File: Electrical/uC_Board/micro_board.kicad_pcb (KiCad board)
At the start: 2 copper layers, 45 x 18 mm, 27 parts, among them J1 card_edge_6p, SW1 SW_Push, U1 ATmega328PB-AU, U2 ArdStripNano, U3 CSTNE16M0V530000R0, U4 AD8620, U5 LM1117MPX-5.0

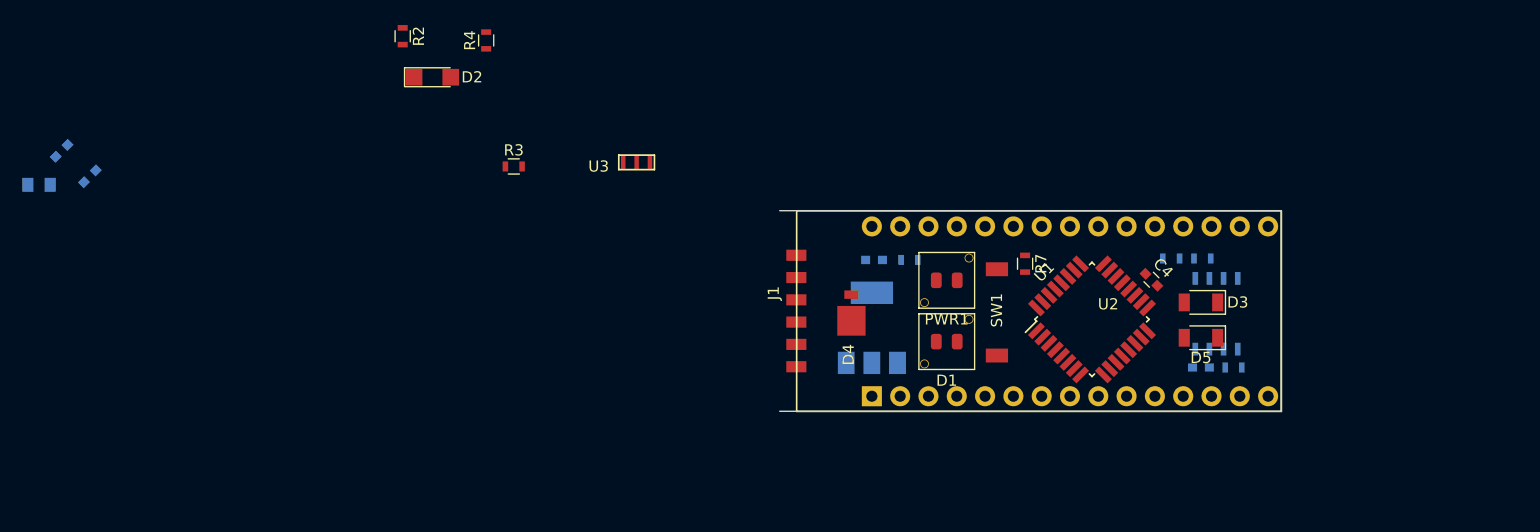
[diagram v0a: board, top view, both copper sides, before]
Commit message: forgot to save earlier
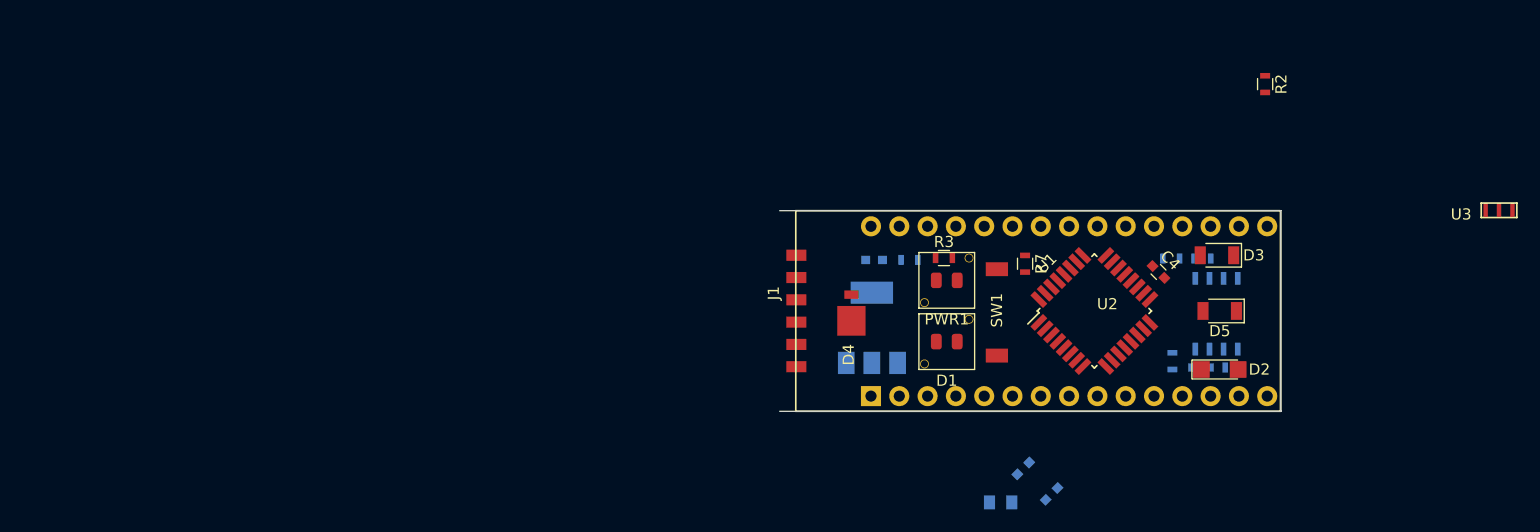
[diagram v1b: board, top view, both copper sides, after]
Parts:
- R4: moved to B.Cu
- moved C1 90.9 mm to (124.4, 116.4)
- moved C2 90.9 mm to (119.8, 117.2)
- moved C3 90.9 mm to (121.9, 114.1)
- moved R2 77.5 mm to (143.6, 79.6)
- moved U3 77.5 mm to (163.0, 91.6)
- moved D2 75.4 mm to (139.5, 105.2)
- moved R4 68.0 mm to (135.2, 104.5), turned to 270 degrees
- moved R3 39.5 mm to (114.8, 95.2)
- moved D3 4.47 mm to (139.2, 95.0)
- moved D5 2.94 mm to (139.5, 100.0)
- moved C4 0.94 mm to (134.0, 96.5)
- moved U1 0.78 mm to (128.2, 100.0)
- moved U2 0.08 mm to (147.7, 91.0)
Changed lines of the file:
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@@
   (general
     (thickness 1.6)
-    (drawings 5)
+    (drawings 6)
     (tracks 0)
     (zones 0)
@@
   (layers
     (0 F.Cu signal)
-    (31 B.Cu signal)
+    (31 B.Cu signal hide)
     (32 B.Adhes user)
     (33 F.Adhes user)
@@
     (add_net VCC)
   )
-  (module hodgkin:LED_0805_LightPipe (layer F.Cu)
+  (module hodgkin:LED_0805_LightPipe locked (layer F.Cu)
     (at 115 97.25 180)
     (descr "LED SMD 1206 (3216 Metric), square (rectangular) end terminal, IPC_7351 nominal, (Body size source: http://www.tortai-tech.com/upload/download/2011102023233369053.pdf), generated with kicad-footprint-generator")
@@
     )
   )
-  (module hodgkin:LED_0805_LightPipe (layer F.Cu)
+  (module hodgkin:LED_0805_LightPipe locked (layer F.Cu)
     (at 115 102.75 180)
     (descr "LED SMD 1206 (3216 Metric), square (rectangular) end terminal, IPC_7351 nominal, (Body size source: http://www.tortai-tech.com/upload/download/2011102023233369053.pdf), generated with kicad-footprint-generator")
@@
   )
   (module hodgkin:CSTNE16M0V530000R0 (layer F.Cu)
-    (at 85.564999 87.313)
+    (at 162.964999 91.613)
     (fp_text reference U3 (at -1.802999 -0.285) (layer F.SilkS)
       (effects (font (size 1 1) (thickness 0.15)))
@@
       (net 31 "Net-(U1-Pad8)"))
   )
-  (module hodgkin:PTS636-G-2.5-NoGND (layer F.Cu)
+  (module hodgkin:PTS636-G-2.5-NoGND locked (layer F.Cu)
     (at 119.5 104 90)
     (fp_text reference SW1 (at 4.064 0 90) (layer F.SilkS)
@@
     )
   )
-  (module Resistors_SMD:R_0603 (layer F.Cu)
-    (at 73.666 75.722 90)
+  (module Resistors_SMD:R_0603 (layer B.Cu)
+    (at 135.25 104.5 270)
     (descr "Resistor SMD 0603, reflow soldering, Vishay (see dcrcw.pdf)")
     (tags "resistor 0603")
     (attr smd)
-    (fp_text reference R4 (at 0 -1.45 90) (layer F.SilkS)
-      (effects (font (size 1 1) (thickness 0.15)))
-    )
-    (fp_text value R (at 0 1.5 90) (layer F.Fab)
-      (effects (font (size 1 1) (thickness 0.15)))
-    )
-    (fp_text user %R (at 0 0 90) (layer F.Fab)
-      (effects (font (size 0.4 0.4) (thickness 0.075)))
-    )
-    (fp_line (start -0.8 0.4) (end -0.8 -0.4) (layer F.Fab) (width 0.1))
-    (fp_line (start 0.8 0.4) (end -0.8 0.4) (layer F.Fab) (width 0.1))
-    (fp_line (start 0.8 -0.4) (end 0.8 0.4) (layer F.Fab) (width 0.1))
-    (fp_line (start -0.8 -0.4) (end 0.8 -0.4) (layer F.Fab) (width 0.1))
-    (fp_line (start 0.5 0.68) (end -0.5 0.68) (layer F.SilkS) (width 0.12))
-    (fp_line (start -0.5 -0.68) (end 0.5 -0.68) (layer F.SilkS) (width 0.12))
-    (fp_line (start -1.25 -0.7) (end 1.25 -0.7) (layer F.CrtYd) (width 0.05))
-    (fp_line (start -1.25 -0.7) (end -1.25 0.7) (layer F.CrtYd) (width 0.05))
-    (fp_line (start 1.25 0.7) (end 1.25 -0.7) (layer F.CrtYd) (width 0.05))
-    (fp_line (start 1.25 0.7) (end -1.25 0.7) (layer F.CrtYd) (width 0.05))
-    (pad 1 smd rect (at -0.75 0 90) (size 0.5 0.9) (layers F.Cu F.Paste F.Mask)
+    (fp_text reference R4 (at 0 1.45 270) (layer B.SilkS)
+      (effects (font (size 1 1) (thickness 0.15)) (justify mirror))
+    )
+    (fp_text value R (at 0 -1.5 270) (layer B.Fab)
+      (effects (font (size 1 1) (thickness 0.15)) (justify mirror))
+    )
+    (fp_text user %R (at 0 0 270) (layer B.Fab)
+      (effects (font (size 0.4 0.4) (thickness 0.075)) (justify mirror))
+    )
+    (fp_line (start -0.8 -0.4) (end -0.8 0.4) (layer B.Fab) (width 0.1))
+    (fp_line (start 0.8 -0.4) (end -0.8 -0.4) (layer B.Fab) (width 0.1))
+    (fp_line (start 0.8 0.4) (end 0.8 -0.4) (layer B.Fab) (width 0.1))
+    (fp_line (start -0.8 0.4) (end 0.8 0.4) (layer B.Fab) (width 0.1))
+    (fp_line (start 0.5 -0.68) (end -0.5 -0.68) (layer B.SilkS) (width 0.12))
+    (fp_line (start -0.5 0.68) (end 0.5 0.68) (layer B.SilkS) (width 0.12))
+    (fp_line (start -1.25 0.7) (end 1.25 0.7) (layer B.CrtYd) (width 0.05))
+    (fp_line (start -1.25 0.7) (end -1.25 -0.7) (layer B.CrtYd) (width 0.05))
+    (fp_line (start 1.25 -0.7) (end 1.25 0.7) (layer B.CrtYd) (width 0.05))
+    (fp_line (start 1.25 -0.7) (end -1.25 -0.7) (layer B.CrtYd) (width 0.05))
+    (pad 1 smd rect (at -0.75 0 270) (size 0.5 0.9) (layers B.Cu B.Paste B.Mask)
       (net 4 "Net-(D2-Pad2)"))
-    (pad 2 smd rect (at 0.75 0 90) (size 0.5 0.9) (layers F.Cu F.Paste F.Mask)
+    (pad 2 smd rect (at 0.75 0 270) (size 0.5 0.9) (layers B.Cu B.Paste B.Mask)
       (net 14 /TX))
     (model ${KISYS3DMOD}/Resistors_SMD.3dshapes/R_0603.wrl
@@
   )
   (module Resistors_SMD:R_0603 (layer F.Cu)
-    (at 76.142 87.028)
+    (at 114.75 95.25)
     (descr "Resistor SMD 0603, reflow soldering, Vishay (see dcrcw.pdf)")
     (tags "resistor 0603")
@@
   )
   (module Resistors_SMD:R_0603 (layer F.Cu)
-    (at 66.173 75.341 270)
+    (at 143.573 79.641 270)
     (descr "Resistor SMD 0603, reflow soldering, Vishay (see dcrcw.pdf)")
     (tags "resistor 0603")
@@
   )
   (module Diodes_SMD:D_1206 (layer F.Cu)
-    (at 137.813 102.405 180)
+    (at 139.5 100 180)
     (descr "Diode SMD 1206, reflow soldering http://datasheets.avx.com/schottky.pdf")
     (tags "Diode 1206")
@@
   )
   (module Capacitors_SMD:C_0603 (layer F.Cu)
-    (at 133.368 97.198 315)
+    (at 134 96.5 315)
     (descr "Capacitor SMD 0603, reflow soldering, AVX (see smccp.pdf)")
     (tags "capacitor 0603")
@@
   )
   (module Capacitors_SMD:C_0603 (layer B.Cu)
-    (at 35.566 85.628 225)
+    (at 121.866 114.128 225)
     (descr "Capacitor SMD 0603, reflow soldering, AVX (see smccp.pdf)")
     (tags "capacitor 0603")
@@
   )
   (module Capacitors_SMD:C_0805 (layer B.Cu)
-    (at 33.534 88.676)
+    (at 119.834 117.176)
     (descr "Capacitor SMD 0805, reflow soldering, AVX (see smccp.pdf)")
     (tags "capacitor 0805")
@@
   )
   (module Capacitors_SMD:C_0603 (layer B.Cu)
-    (at 38.106 87.914 225)
+    (at 124.406 116.414 225)
     (descr "Capacitor SMD 0603, reflow soldering, AVX (see smccp.pdf)")
     (tags "capacitor 0603")
@@
   )
   (module Diodes_SMD:D_1206 (layer F.Cu)
-    (at 137.813 99.23 180)
+    (at 139.25 95 180)
     (descr "Diode SMD 1206, reflow soldering http://datasheets.avx.com/schottky.pdf")
     (tags "Diode 1206")
@@
   )
   (module LEDs:LED_1206 (layer F.Cu)
-    (at 68.84 79.024)
+    (at 139.5 105.25)
     (descr "LED 1206 smd package")
     (tags "LED led 1206 SMD smd SMT smt smdled SMDLED smtled SMTLED")
@@
     )
   )
-  (module hodgkin:ArdNanoStrip (layer F.Cu)
-    (at 147.78 91.01 180)
+  (module hodgkin:ArdNanoStrip locked (layer F.Cu)
+    (at 147.7 91 180)
     (descr "Arduino Nano, http://www.mouser.com/pdfdocs/Gravitech_Arduino_Nano3_0.pdf")
     (tags "Arduino Nano")
@@
   )
   (module hodgkin:TQFP-32_7x7mm_P0.8mm (layer F.Cu)
-    (at 128.034 100.754 45)
+    (at 128.25 100 45)
     (descr "32-Lead Plastic Thin Quad Flatpack (PT) - 7x7x1.0 mm Body, 2.00 mm [TQFP] (see Microchip Packaging Specification 00000049BS.pdf)")
     (tags "QFP 0.8")
@@
     )
   )
+  (gr_line (start 104.7 91) (end 104.7 109) (layer Dwgs.User) (width 0.15))
   (gr_line (start 100 91) (end 100 109) (layer Dwgs.User) (width 0.15))
   (gr_line (start 94.996 100) (end 152.146 100) (layer Dwgs.User) (width 0.15))
